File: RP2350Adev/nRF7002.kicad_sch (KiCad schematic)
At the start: 8 parts, among them U1 NRF7002-QFAA-R, U4 CX1612DB40000D0WLLCC

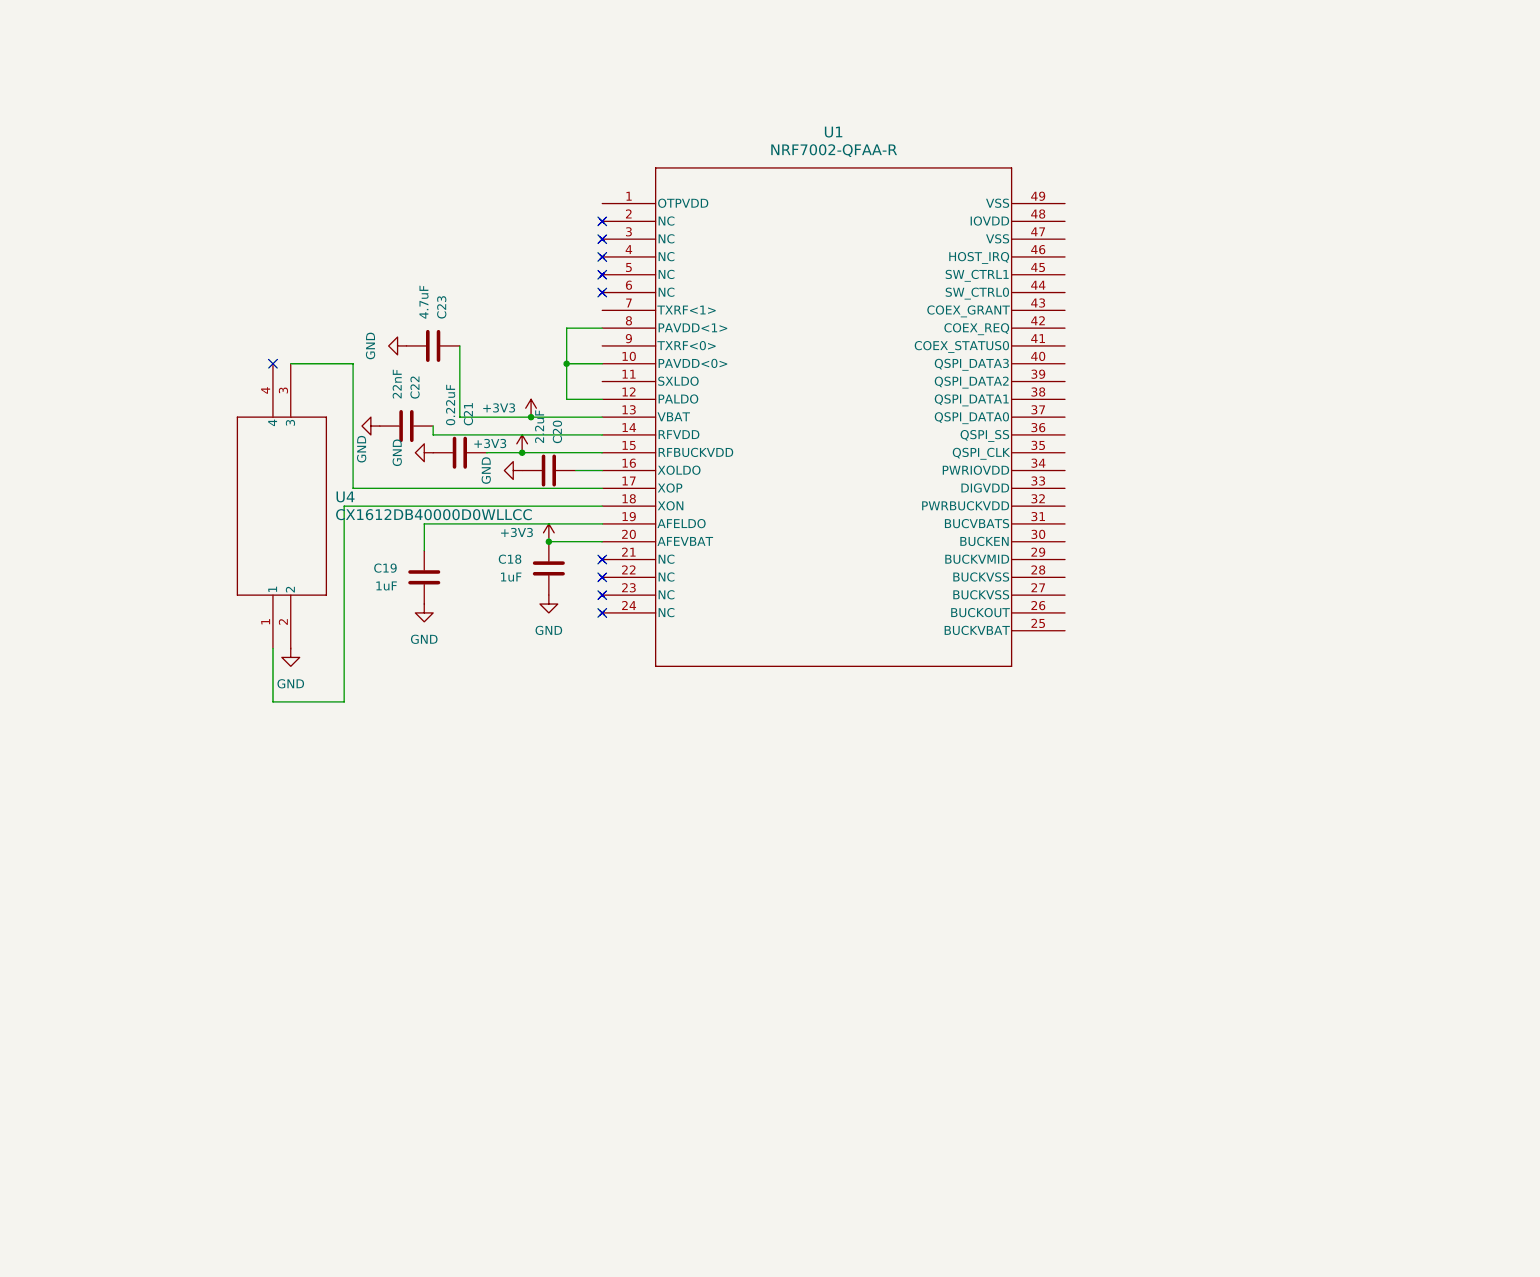
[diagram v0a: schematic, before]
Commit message: add footprints
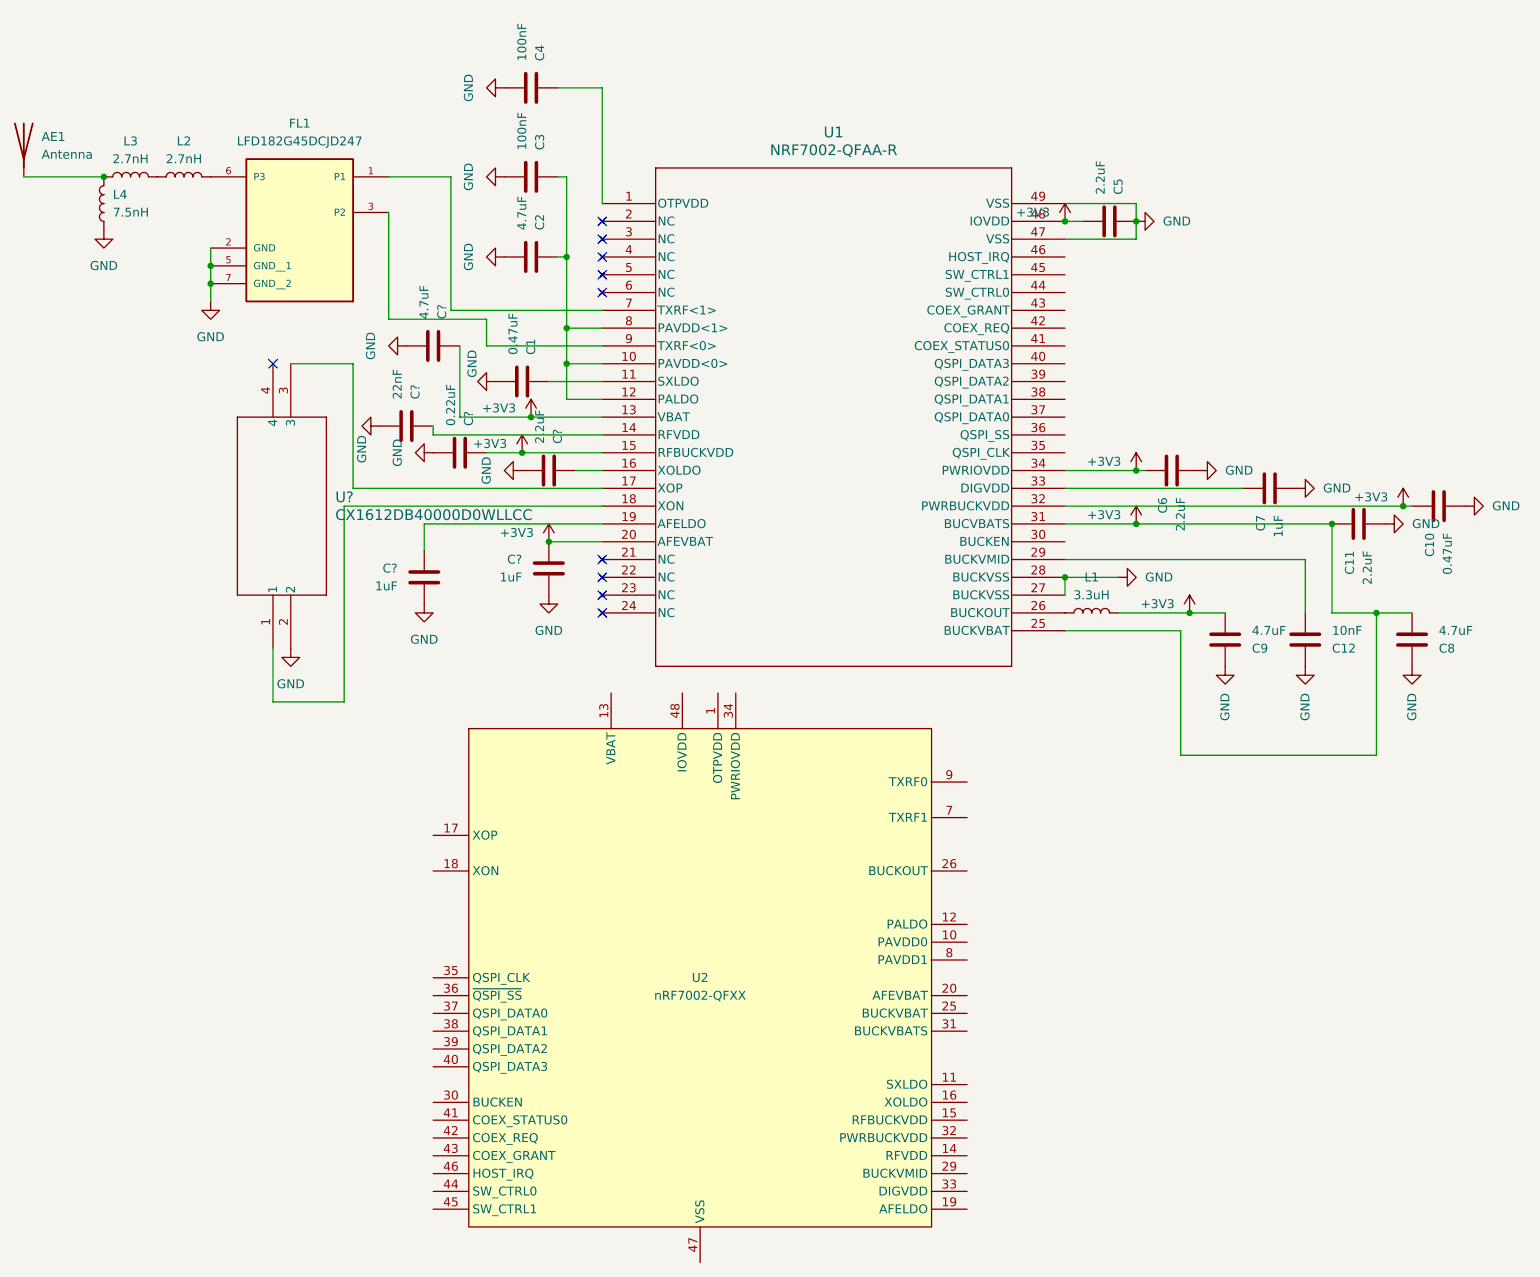
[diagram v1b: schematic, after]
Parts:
- added AE1: Antenna, symbol Device:Antenna
- added C1, C10: 0.47uF, Resistor_SMD:R_0402_1005Metric, symbol Device:C
- added C11, C5, C6: 2.2uF, Resistor_SMD:R_0402_1005Metric, symbol Device:C
- added C12: 10nF, Resistor_SMD:R_0402_1005Metric, symbol Device:C
- added C2, C8, C9: 4.7uF, Resistor_SMD:R_0402_1005Metric, symbol Device:C
- added C3, C4: 100nF, Resistor_SMD:R_0402_1005Metric, symbol Device:C
- added C7: 1uF, Resistor_SMD:R_0402_1005Metric, symbol Device:C
- added FL1: LFD182G45DCJD247, LFD182G45DCJD247:FIL_LFD182G45DCJD247, symbol LFD182G45DCJD247:LFD182G45DCJD247
- added L1: 3.3uH, Inductor_SMD:L_0805_2012Metric, symbol Device:L
- added L2, L3: 2.7nH, Inductor_SMD:L_0805_2012Metric, symbol Device:L
- added L4: 7.5nH, Inductor_SMD:L_0805_2012Metric, symbol Device:L
- added U2: nRF7002-QFXX, Package_DFN_QFN:QFN-48-1EP_6x6mm_P0.4mm_EP4.6x4.6mm_ThermalVias, symbol PCM_nordic-lib-kicad-nrf7:nRF7002-QFXX
- renumbered C20 to C?, C19 to C?, C23 to C?, C21 to C?, C22 to C?, C18 to C?, U4 to U?
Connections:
- net +3V3: now also U1.25 (BUCKVBAT), U1.31 (BUCVBATS), U1.32 (PWRBUCKVDD), U1.34 (PWRIOVDD), U1.48 (IOVDD), C10.2, C11.2, C5.1, C6.2, C8.1, C9.1, L1.2
- net GND: now also U1.27 (BUCKVSS), U1.28 (BUCKVSS), U1.47 (VSS), U1.49 (VSS), C1.1, C10.1, C11.1, C12.2, C2.1, C3.1, C4.1, C5.2, C6.1, C7.1, C8.2, C9.2, FL1.2 (GND), FL1.5 (GND__1), FL1.7 (GND__2), L4.1
- net at U1.1 (OTPVDD): now also C4.2
- net at U1.10 (PAVDD<0>), U1.12 (PALDO), U1.8 (PAVDD<1>): now also C2.2, C3.2
- net at U1.11 (SXLDO): now also C1.2
- net at U1.26 (BUCKOUT): now also L1.1
- net at U1.29 (BUCKVMID): now also C12.1
- net at U1.33 (DIGVDD): now also C7.2
- net at U1.7 (TXRF<1>): now also FL1.1 (P1)
- net at U1.9 (TXRF<0>): now also FL1.3 (P2)
- new net: L2.1, L3.2
- new net: FL1.6 (P3), L2.2
- new net: U2.27 (BUCKVSS), U2.28 (BUCKVSS), U2.47 (VSS), U2.49 (EP)
- new net: AE1.1 (A), L3.1, L4.2
